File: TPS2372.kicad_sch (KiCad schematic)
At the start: 29 parts

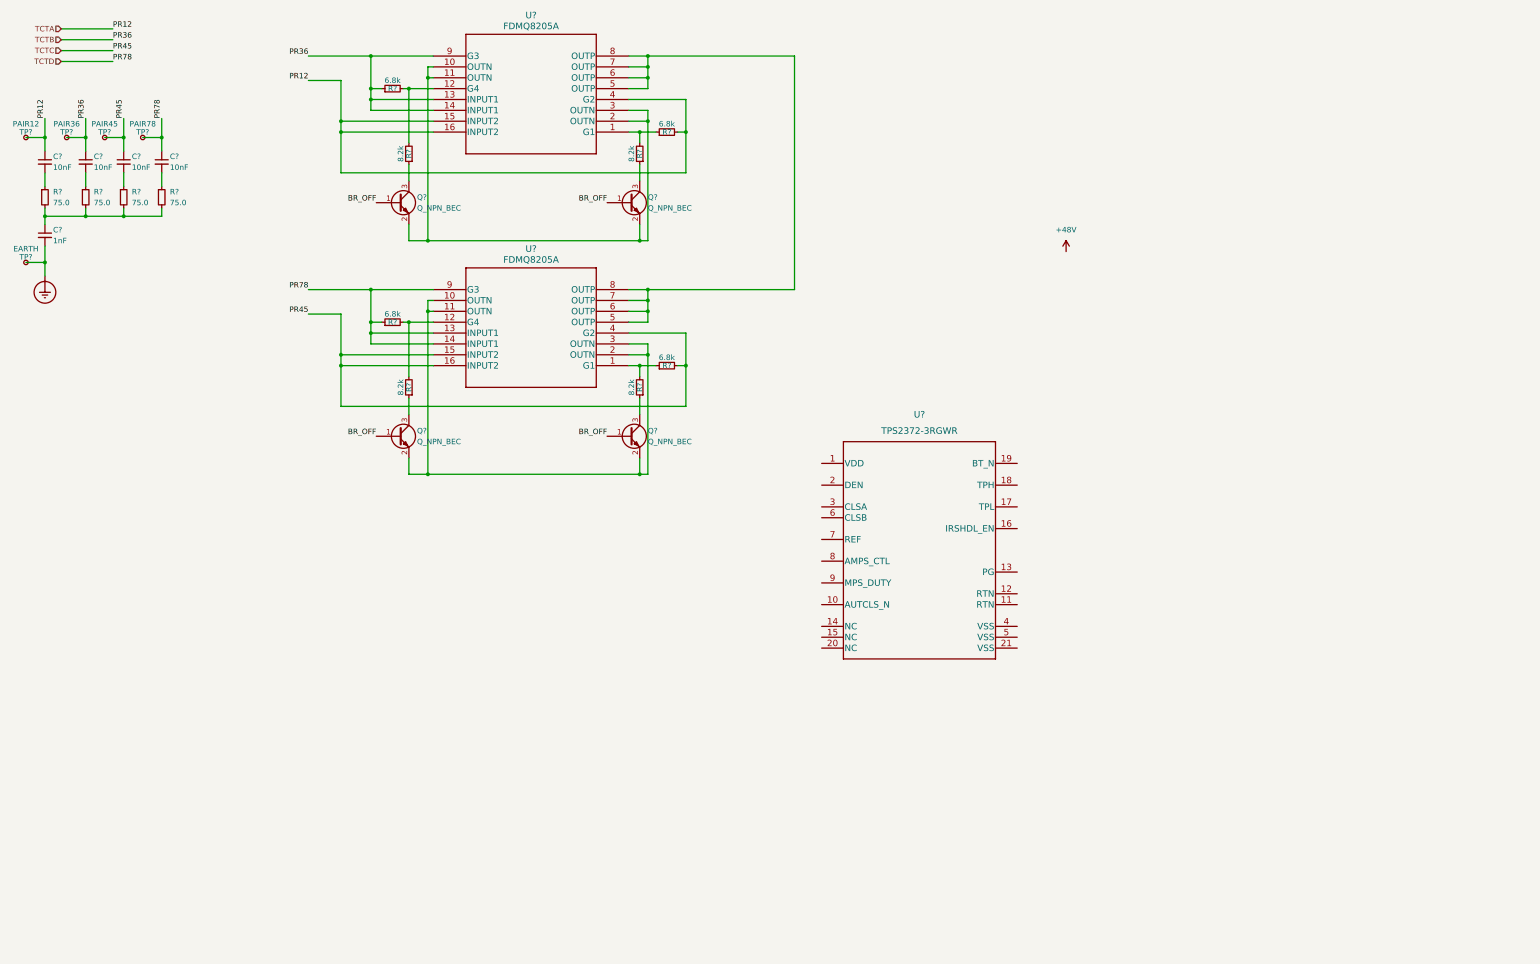
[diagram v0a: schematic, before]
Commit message: tps2372 finish
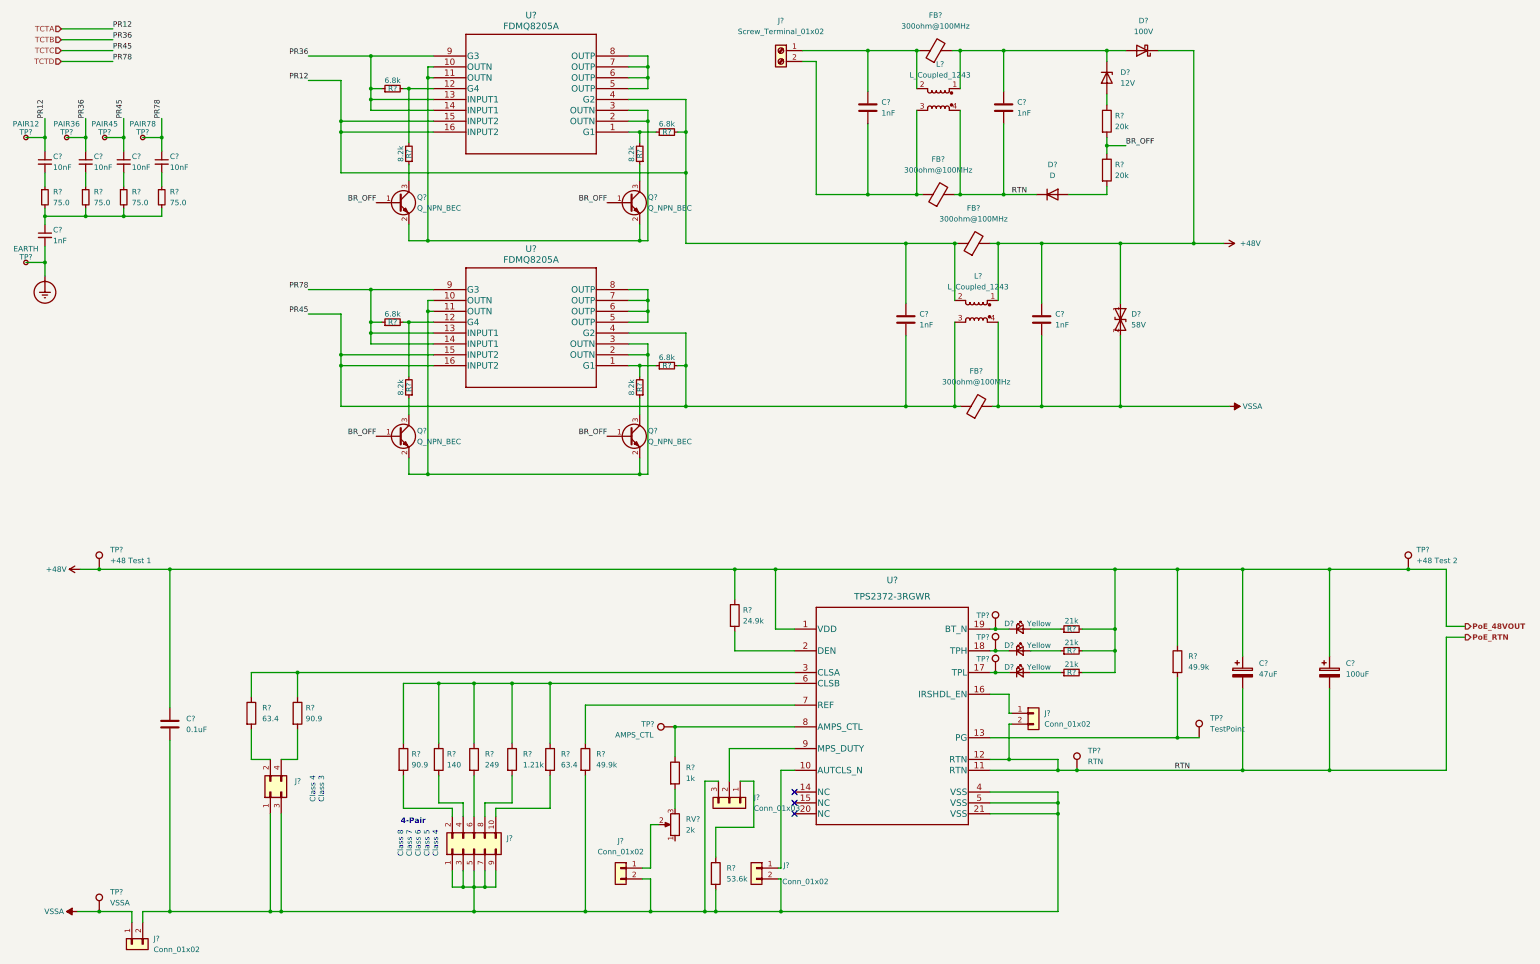
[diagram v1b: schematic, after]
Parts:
- added C? (x4): 1nF, symbol Device:C
- added C?: 0.1uF, symbol Device:C
- added C?: 100uF, symbol Device:C_Polarized
- added C?: 47uF, symbol Device:C_Polarized
- added D?: 58V, symbol Device:D_TVS
- added D? (x3): Yellow, symbol Device:LED_Small
- added D?: D, symbol Device:D
- added D?: 100V, symbol Device:D_Schottky
- added D?: 12V, symbol Device:D_Zener
- added FB? (x4): 300ohm@100MHz, symbol Device:FerriteBead
- added J? (x3): Conn_01x02, TestPoint:TestPoint_2Pads_Pitch2.54mm_Drill0.8mm, symbol Connector_Generic:Conn_01x02
- added J?: Conn_01x03, symbol Connector_Generic:Conn_01x03
- added J?: Conn_02x05_Odd_Even, symbol Connector_Generic:Conn_02x05_Odd_Even
- added J?: Conn_02x02_Odd_Even, symbol Connector_Generic:Conn_02x02_Odd_Even
- added J?: Screw_Terminal_01x02, symbol Connector:Screw_Terminal_01x02
- added J?: Conn_01x02, symbol Connector_Generic:Conn_01x02
- added L? (x2): L_Coupled_1243, symbol Device:L_Coupled_1243
- added R?: 249, symbol Device:R
- added R?: 24.9k, symbol Device:R
- added R? (x3): 21k, symbol Device:R_Small
- added R? (x2): 49.9k, symbol Device:R
- added R?: 1k, symbol Device:R
- added R? (x2): 20k, symbol Device:R
- added R? (x2): 90.9, symbol Device:R
- added R?: 140, symbol Device:R
- added R? (x2): 63.4, symbol Device:R
- added R?: 53.6k, symbol Device:R
- added R?: 1.21k, symbol Device:R
- added RV?: 2k, symbol Device:R_Potentiometer
- added TP?: VSSA, symbol Connector:TestPoint
- added TP?: +48 Test 2, symbol Connector:TestPoint
- added TP?: AMPS_CTL, symbol Connector:TestPoint
- added TP? (x4): TestPoint, symbol Connector:TestPoint
- added TP?: RTN, symbol Connector:TestPoint
- added TP?: +48 Test 1, symbol Connector:TestPoint
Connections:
- net +48V: now also U?.1 (VDD), C?.1, C?.1, C?.1, C?.1, D?.1 (A1), D?.1 (K), FB?.2, L?.1, R?.1, R?.1, R?.2, R?.2, R?.2, TP?.1, TP?.1
- net BR_OFF: now also R?.1, R?.2
- net TCTA: now also C?.1, FB?.1, L?.2
- net TCTC: now also C?.2, FB?.1, L?.3
- net at U?.10 (AUTCLS_N): now also J?.1 (Pin_1)
- net PoE_RTN: now reaches U?.11 (RTN)
- net PoE_RTN: now also U?.12 (RTN), C?.2, C?.2, C?.2, D?.1 (K), FB?.2, J?.2 (Pin_2), L?.4, TP?.1
- net at U?.13 (PG): now also R?.2, TP?.1
- net at U?.16 (IRSHDL_EN): now also J?.1 (Pin_1)
- net at U?.17 (TPL): now also D?.1 (K), TP?.1
- net at U?.18 (TPH): now also D?.1 (K), TP?.1
- net at U?.19 (BT_N): now also D?.1 (K), TP?.1
- net at U?.2 (DEN): now also R?.2
- net at U?.21 (VSS): now also U?.4 (VSS), U?.5 (VSS), C?.2, J?.1 (Pin_1), J?.1 (Pin_1), J?.2 (Pin_2), J?.2 (Pin_2), J?.2 (Pin_2), J?.3 (Pin_3), J?.3 (Pin_3), J?.3 (Pin_3), J?.5 (Pin_5), J?.7 (Pin_7), J?.9 (Pin_9), R?.2, R?.2
- net at U?.3 (CLSA): now also R?.1, R?.1
- net at U?.6 (CLSB): now also R?.1, R?.1, R?.1, R?.1, R?.1
- net at U?.7 (REF): now also R?.1
- net at U?.8 (AMPS_CTL): now also R?.1, TP?.1
- net at U?.9 (MPS_DUTY): now also J?.2 (Pin_2)
- net at U?.5 (OUTP), U?.6 (OUTP), U?.7 (OUTP)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: no longer U?.5 (OUTP), U?.6 (OUTP), U?.7 (OUTP), U?.8 (OUTP)
- new net: J?.6 (Pin_6), R?.2
- new net: C?.2, FB?.1, J?.2 (Pin_2), L?.3
- new net: D?.2 (A), R?.1 (x4)
- new net: J?.1 (Pin_1), RV?.2
- new net: R?.2, RV?.3
- new net: J?.1 (Pin_1), R?.1
- new net: C?.1, D?.1 (K), D?.2 (A), FB?.2, L?.1
- new net: C?.1, FB?.1, J?.1 (Pin_1), L?.2
- new net: U?.5 (OUTP), U?.6 (OUTP), U?.7 (OUTP), U?.8 (OUTP)
- new net: J?.10 (Pin_10), R?.2
- new net: J?.2 (Pin_2), R?.2 (x2)
- new net: J?.4 (Pin_4), R?.2 (x2)
- new net: J?.8 (Pin_8), R?.2
- new net: D?.2 (A), R?.2
- new net VSSA: C?.2, D?.2 (A2), FB?.2, J?.1 (Pin_1), L?.4, TP?.1
- no-connect marks 0 -> 3
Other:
- note added: "4-Pair"
- note added: "Class 4 Class 3"
- note added: "Class 8 Class 7 Class 6 Class 5 Class 4"
- moved on the sheet: U?

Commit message: buck converter init
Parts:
- J?: footprint (none) -> TestPoint:TestPoint_2Pads_Pitch2.54mm_Drill0.8mm
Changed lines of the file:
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@@
       (effects (font (size 1.27 1.27)) (justify right))
     )
-    (property "Footprint" "" (id 2) (at 41.91 234.95 0)
+    (property "Footprint" "TestPoint:TestPoint_2Pads_Pitch2.54mm_Drill0.8mm" (id 2) (at 41.91 234.95 0)
       (effects (font (size 1.27 1.27)) hide)
     )
